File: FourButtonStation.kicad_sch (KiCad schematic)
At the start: 63 parts, among them J1 AC IN, J10 AC IN, J2 External 3V, J3 UART, J4 ADC, J5 Conn_WallSocket, J6 USB_B_Micro, J7 Conn_WallSocket, J8 Conn_WallSocket, J9 Conn_WallSocket, K1 G5LE-1, K2 G5LE-1, K3 G5LE-1, K4 G5LE-1, Q1 MMBT3904, Q3 MMBT3904, SW1 POWER, SW2 RST, SW5 Mode, U1 CH340C, U10 SM4007PL, U11 D882_C9634, U13 AMS1117-3_3, U2 radio-receiver, U3 ESP-07, U4 SM4007PL, U5 D882_C9634, U6 SM4007PL, U7 D882_C9634, U8 SM4007PL, U9 D882_C9634

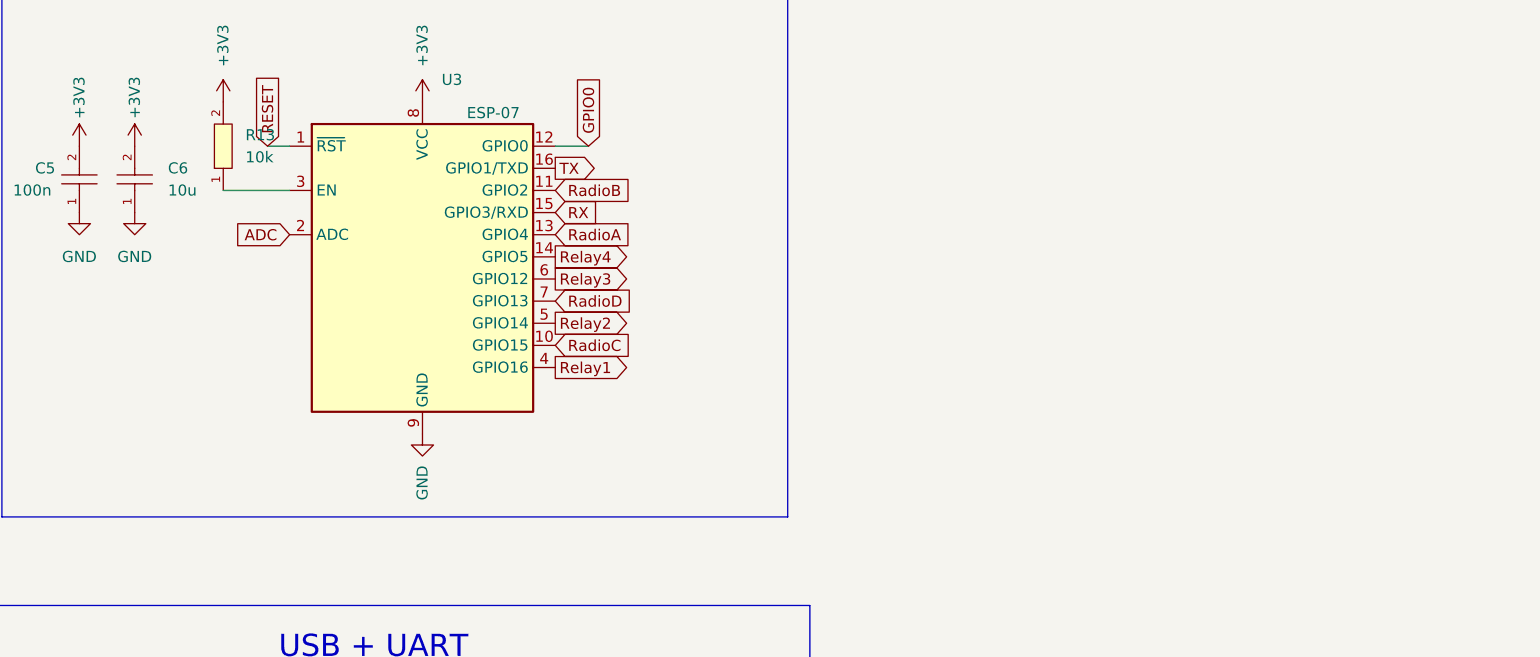
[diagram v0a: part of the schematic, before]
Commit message: Update schematic
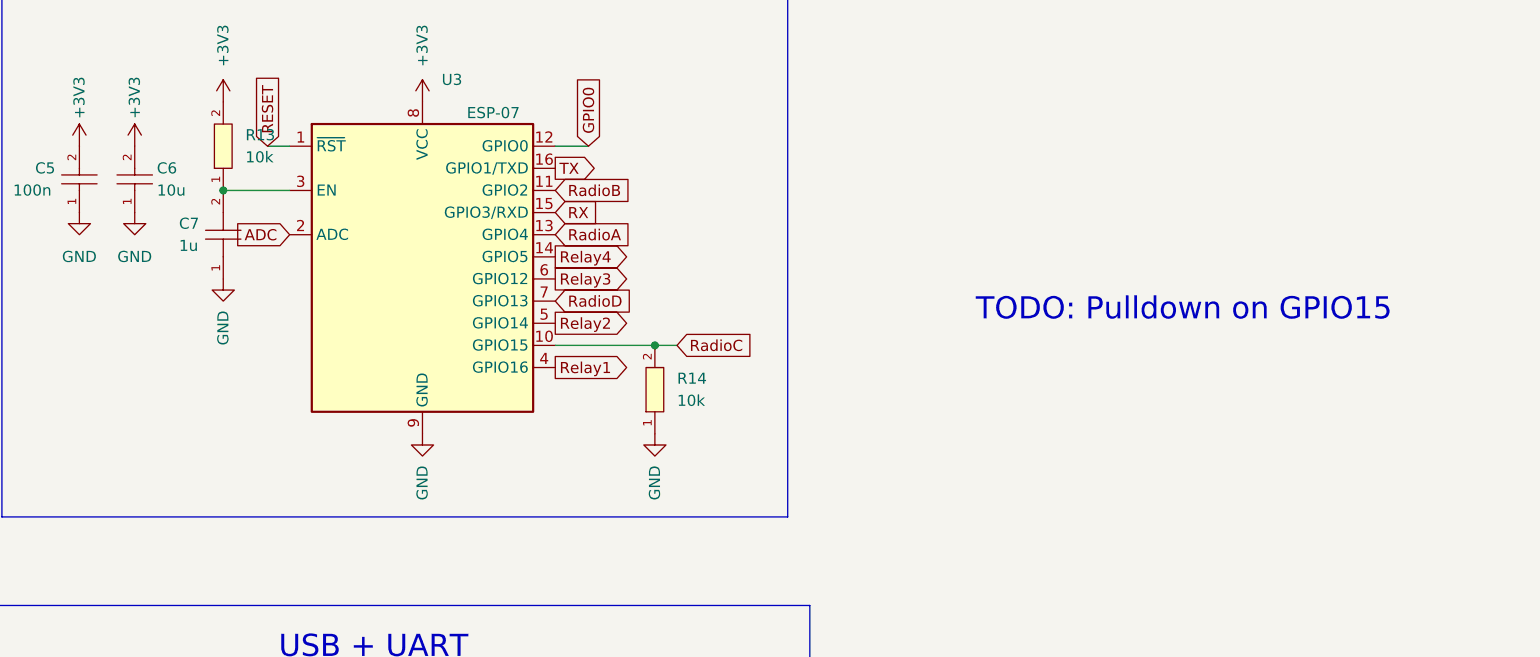
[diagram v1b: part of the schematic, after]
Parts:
- added C7: 1u, jlc_footprints:C0603, symbol jlc_symbols:CL10A105KB8NNNC
- added R14: 10k, jlc_footprints:R0603, symbol jlc_symbols:0603WAF1002T5E
- J1: footprint c8-inlet:c8-inlet -> c8-inlet:c8-inlet-old
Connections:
- net GND: now also C7.1, R14.1
- net RadioC: now also R14.2
- net at R13.1, U3.3 (EN): now also C7.2
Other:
- note added: "TODO: Pulldown on GPIO15"
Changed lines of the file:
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@@
   (junction (at 121.285 72.39) (diameter 0) (color 0 0 0 0)
   )
+  (junction (at 267.97 59.69) (diameter 0) (color 0 0 0 0)
+  )
   (junction (at 43.815 159.385) (diameter 0) (color 0 0 0 0)
   )
@@
   (junction (at 34.925 90.805) (diameter 0) (color 0 0 0 0)
   )
+  (junction (at 218.44 41.91) (diameter 0) (color 0 0 0 0)
+  )
   (junction (at 100.965 38.735) (diameter 0) (color 0 0 0 0)
   )
@@
     (stroke (width 0) (type default))
   )
+  (wire (pts (xy 267.97 59.69) (xy 270.51 59.69))
+    (stroke (width 0) (type default))
+  )
   (wire (pts (xy 43.815 69.215) (xy 43.815 70.485))
     (stroke (width 0) (type default))
@@
     (stroke (width 0) (type default))
   )
+  (wire (pts (xy 256.54 59.69) (xy 267.97 59.69))
+    (stroke (width 0) (type default))
+  )
   (wire (pts (xy 117.475 38.735) (xy 123.825 38.735))
     (stroke (width 0) (type default))
@@
     (effects (font (size 2.54 2.54)) (justify left bottom))
   )
+  (text "TODO: Pulldown on GPIO15\n" (at 304.8 57.15 0)
+    (effects (font (size 2.54 2.54)) (justify left bottom))
+  )
   (label "Nullleiter" (at 66.675 93.345 180) (fields_autoplaced)
     (effects (font (size 1.27 1.27)) (justify right bottom))
@@
     )
   )
-  (global_label "RadioC" (shape input) (at 256.54 59.69 0) (fields_autoplaced)
+  (global_label "RadioC" (shape input) (at 270.51 59.69 0) (fields_autoplaced)
     (effects (font (size 1.27 1.27)) (justify left))
-    (property "Intersheetrefs" "${INTERSHEET_REFS}" (at 265.545 59.7694 0)
+    (property "Intersheetrefs" "${INTERSHEET_REFS}" (at 279.515 59.7694 0)
       (effects (font (size 1.27 1.27)) (justify left) hide)
     )
@@
     )
   )
+  (symbol (lib_id "power:GND") (at 218.44 52.07 0) (unit 1)
+    (in_bom yes) (on_board yes) (dnp no)
+    (property "Reference" "#PWR042" (at 218.44 58.42 0)
+      (effects (font (size 1.27 1.27)) hide)
+    )
+    (property "Value" "GND" (at 218.44 59.69 90)
+      (effects (font (size 1.27 1.27)) (justify left))
+    )
+    (property "Footprint" "" (at 218.44 52.07 0)
+      (effects (font (size 1.27 1.27)) hide)
+    )
+    (property "Datasheet" "" (at 218.44 52.07 0)
+      (effects (font (size 1.27 1.27)) hide)
+    )
+    (pin "1")
+    (instances
+      (project "FourButtonStation"
+        (path "/fe8954b5-d30a-4533-a19e-bff77a7cd4d5"
+          (reference "#PWR042") (unit 1)
+        )
+      )
+    )
+  )
   (symbol (lib_id "Graphic:SYM_Flash_XLarge") (at 80.645 110.49 0) (unit 1)
     (in_bom no) (on_board no) (dnp no) (fields_autoplaced)
@@
     )
   )
+  (symbol (lib_id "jlc_symbols:0603WAF1002T5E") (at 267.97 64.77 90) (unit 1)
+    (in_bom yes) (on_board yes) (dnp no) (fields_autoplaced)
+    (property "Reference" "R14" (at 270.51 63.5 90)
+      (effects (font (size 1.27 1.27)) (justify right))
+    )
+    (property "Value" "10k" (at 270.51 66.04 90)
+      (effects (font (size 1.27 1.27)) (justify right))
+    )
+    (property "Footprint" "jlc_footprints:R0603" (at 278.13 64.77 0)
+      (effects (font (size 1.27 1.27) italic) hide)
+    )
+    (property "Datasheet" "https://www.mouser.in/datasheet/2/447/PYu_RT_1_to_0_01_RoHS_L_11-1669912.pdf" (at 267.843 67.056 0)
+      (effects (font (size 1.27 1.27)) (justify left) hide)
+    )
+    (property "LCSC" "C25804" (at 267.97 64.77 0)
+      (effects (font (size 1.27 1.27)) hide)
+    )
+    (pin "1")
+    (pin "2")
+    (instances
+      (project "FourButtonStation"
+        (path "/fe8954b5-d30a-4533-a19e-bff77a7cd4d5"
+          (reference "R14") (unit 1)
+        )
+      )
+    )
+  )
   (symbol (lib_id "Transistor_BJT:MMBT3904") (at 254 127.635 180) (unit 1)
     (in_bom yes) (on_board yes) (dnp no) (fields_autoplaced)
@@
   )
   (symbol (lib_id "CL05A106MQ5NUNC:CL05A106MQ5NUNC") (at 208.28 40.64 90) (unit 1)
-    (in_bom yes) (on_board yes) (dnp no) (fields_autoplaced)
-    (property "Reference" "C6" (at 212.09 39.3699 90)
+    (in_bom yes) (on_board yes) (dnp no)
+    (property "Reference" "C6" (at 210.82 39.37 90)
       (effects (font (size 1.27 1.27)) (justify right))
     )
-    (property "Value" "10u" (at 212.09 41.9099 90)
+    (property "Value" "10u" (at 210.82 41.91 90)
       (effects (font (size 1.27 1.27)) (justify right))
     )
@@
     )
   )
+  (symbol (lib_id "jlc_symbols:CL10A105KB8NNNC") (at 218.44 46.99 90) (unit 1)
+    (in_bom yes) (on_board yes) (dnp no)
+    (property "Reference" "C7" (at 213.36 45.72 90)
+      (effects (font (size 1.27 1.27)) (justify right))
+    )
+    (property "Value" "1u" (at 213.36 48.26 90)
+      (effects (font (size 1.27 1.27)) (justify right))
+    )
+    (property "Footprint" "jlc_footprints:C0603" (at 228.6 46.99 0)
+      (effects (font (size 1.27 1.27) italic) hide)
+    )
+    (property "Datasheet" "https://item.szlcsc.com/362304.html" (at 218.313 49.276 0)
+      (effects (font (size 1.27 1.27)) (justify left) hide)
+    )
+    (property "LCSC" "C15849" (at 218.44 46.99 0)
+      (effects (font (size 1.27 1.27)) hide)
+    )
+    (pin "2")
+    (pin "1")
+    (instances
+      (project "FourButtonStation"
+        (path "/fe8954b5-d30a-4533-a19e-bff77a7cd4d5"
+          (reference "C7") (unit 1)
+        )
+      )
+    )
+  )
   (symbol (lib_id "jlc_symbols:SM4007PL") (at 34.925 168.275 270) (unit 1)
     (in_bom yes) (on_board yes) (dnp no)
@@
       (effects (font (size 1.27 1.27)) (justify right))
     )
-    (property "Footprint" "c8-inlet:c8-inlet" (at 117.1194 63.1952 0)
+    (property "Footprint" "c8-inlet:c8-inlet-old" (at 117.1194 63.1952 0)
       (effects (font (size 1.27 1.27)) hide)
     )
@@
         )
       )
+    )
+  )
+  (symbol (lib_id "power:GND") (at 267.97 69.85 0) (unit 1)
+    (in_bom yes) (on_board yes) (dnp no)
+    (property "Reference" "#PWR041" (at 267.97 76.2 0)
+      (effects (font (size 1.27 1.27)) hide)
+    )
+    (property "Value" "GND" (at 267.97 77.47 90)
+      (effects (font (size 1.27 1.27)) (justify left))
+    )
+    (property "Footprint" "" (at 267.97 69.85 0)
+      (effects (font (size 1.27 1.27)) hide)
+    )
+    (property "Datasheet" "" (at 267.97 69.85 0)
+      (effects (font (size 1.27 1.27)) hide)
+    )
+    (pin "1")
+    (instances
+      (project "FourButtonStation"
+        (path "/fe8954b5-d30a-4533-a19e-bff77a7cd4d5"
+          (reference "#PWR041") (unit 1)
+        )
+      )
